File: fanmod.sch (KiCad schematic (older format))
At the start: 6 parts, among them J1 FAN_IN, J2 FAN_OUT, J4 COMM

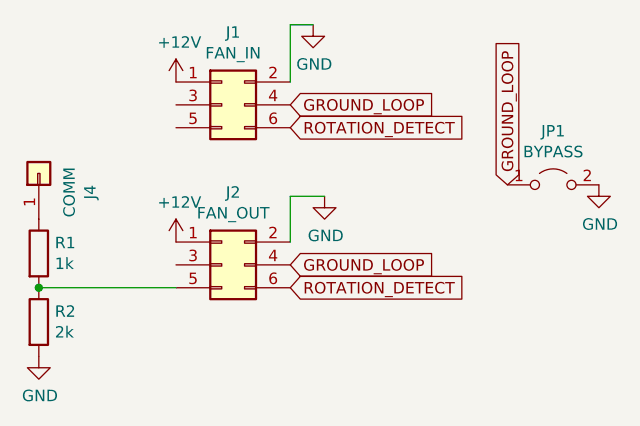
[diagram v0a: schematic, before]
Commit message: board v2.0
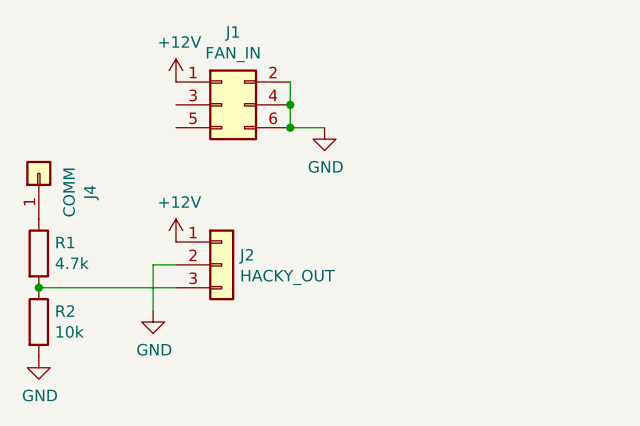
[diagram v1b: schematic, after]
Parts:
- removed J2: FAN_OUT, Connector_PinHeader_2.00mm:PinHeader_2x03_P2.00mm_Vertical_SMD, symbol Connector_Generic:Conn_02x03_Odd_Even
- removed JP1: BYPASS, Jumper:SolderJumper-2_P1.3mm_Open_RoundedPad1.0x1.5mm, symbol Jumper:Jumper_2_Open
- added J2: HACKY_OUT, Connector_PinHeader_2.00mm:PinHeader_1x03_P2.00mm_Vertical, symbol Connector_Generic:Conn_01x03
- J1: footprint Connector_PinSocket_2.00mm:PinSocket_2x03_P2.00mm_Vertical_SMD -> Connector_PinSocket_2.00mm:PinSocket_2x03_P2.00mm_Vertical
- R1: value 1k -> 4.7k
- R2: value 2k -> 10k
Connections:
- net GROUND_LOOP is gone; now on net GND: J1.4 (Pin_4)
- net ROTATION_DETECT is gone; now on net GND: J1.6 (Pin_6)
- net +12V: now also J2.1 (Pin_1)
- net GND: now also J2.2 (Pin_2)
- net at R1.2, R2.1: now also J2.3 (Pin_3)
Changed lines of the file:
@@
 $EndDescr
-$Comp
-L Connector_Generic:Conn_02x03_Odd_Even J2
-U 1 1 5E9E1E9C
-P 5350 3000
-F 0 "J2" H 5400 3317 50  0000 C CNN
-F 1 "FAN_OUT" H 5400 3226 50  0000 C CNN
-F 2 "Connector_PinHeader_2.00mm:PinHeader_2x03_P2.00mm_Vertical_SMD" H 5350 3000 50  0001 C CNN
-F 3 "~" H 5350 3000 50  0001 C CNN
-	1    5350 3000
-	1    0    0    -1
-$EndComp
-Wire Wire Line
-	5650 2700 5800 2700
-Wire Wire Line
-	5650 2900 5650 2700
-$Comp
-L power:GND #PWR0106
-U 1 1 5E9D0844
-P 5800 2700
-F 0 "#PWR0106" H 5800 2450 50  0001 C CNN
-F 1 "GND" H 5805 2527 50  0000 C CNN
-F 2 "" H 5800 2700 50  0001 C CNN
-F 3 "" H 5800 2700 50  0001 C CNN
-	1    5800 2700
-	1    0    0    -1
-$EndComp
 $Comp
 L power:+12V #PWR0105
@@
 	1    0    0    -1
 $EndComp
-Text GLabel 5650 3100 2    50   Input ~ 0
-ROTATION_DETECT
-Text GLabel 5650 2300 2    50   Input ~ 0
-GROUND_LOOP
-Text GLabel 5650 2400 2    50   Input ~ 0
-ROTATION_DETECT
-Wire Wire Line
-	5650 1950 5650 2200
 $Comp
 L Connector_Generic:Conn_02x03_Odd_Even J1
@@
 F 0 "J1" H 5400 2617 50  0000 C CNN
 F 1 "FAN_IN" H 5400 2526 50  0000 C CNN
-F 2 "Connector_PinSocket_2.00mm:PinSocket_2x03_P2.00mm_Vertical_SMD" H 5350 2300 50  0001 C CNN
+F 2 "Connector_PinSocket_2.00mm:PinSocket_2x03_P2.00mm_Vertical" H 5350 2300 50  0001 C CNN
 F 3 "~" H 5350 2300 50  0001 C CNN
 	1    5350 2300
 	1    0    0    -1
 $EndComp
-Wire Wire Line
-	5650 1950 5750 1950
 $Comp
 L power:GND #PWR0104
 U 1 1 5E9CC741
-P 5750 1950
-F 0 "#PWR0104" H 5750 1700 50  0001 C CNN
-F 1 "GND" H 5755 1777 50  0000 C CNN
-F 2 "" H 5750 1950 50  0001 C CNN
-F 3 "" H 5750 1950 50  0001 C CNN
-	1    5750 1950
+P 5800 2400
+F 0 "#PWR0104" H 5800 2150 50  0001 C CNN
+F 1 "GND" H 5805 2227 50  0000 C CNN
+F 2 "" H 5800 2400 50  0001 C CNN
+F 3 "" H 5800 2400 50  0001 C CNN
+	1    5800 2400
 	1    0    0    -1
 $EndComp
@@
 	0    -1   -1   0
 $EndComp
-Text GLabel 5650 3000 2    50   Input ~ 0
-GROUND_LOOP
-$Comp
-L Jumper:Jumper_2_Open JP1
-U 1 1 5EA1EF21
-P 6800 2650
-F 0 "JP1" H 6800 2885 50  0000 C CNN
-F 1 "BYPASS" H 6800 2794 50  0000 C CNN
-F 2 "Jumper:SolderJumper-2_P1.3mm_Open_RoundedPad1.0x1.5mm" H 6800 2650 50  0001 C CNN
-F 3 "~" H 6800 2650 50  0001 C CNN
-	1    6800 2650
-	1    0    0    -1
-$EndComp
-$Comp
-L power:GND #PWR0101
-U 1 1 5EA1F32A
-P 7000 2650
-F 0 "#PWR0101" H 7000 2400 50  0001 C CNN
-F 1 "GND" H 7005 2477 50  0000 C CNN
-F 2 "" H 7000 2650 50  0001 C CNN
-F 3 "" H 7000 2650 50  0001 C CNN
-	1    7000 2650
-	1    0    0    -1
-$EndComp
-Text GLabel 6600 2650 1    50   Input ~ 0
-GROUND_LOOP
 $Comp
 L Device:R R1
@@
 P 4550 2950
 F 0 "R1" H 4620 2996 50  0000 L CNN
-F 1 "1k" H 4620 2905 50  0000 L CNN
+F 1 "4.7k" H 4620 2905 50  0000 L CNN
 F 2 "Resistor_SMD:R_0603_1608Metric_Pad1.05x0.95mm_HandSolder" V 4480 2950 50  0001 C CNN
 F 3 "~" H 4550 2950 50  0001 C CNN
@@
 P 4550 3250
 F 0 "R2" H 4620 3296 50  0000 L CNN
-F 1 "2k" H 4620 3205 50  0000 L CNN
+F 1 "10k" H 4620 3205 50  0000 L CNN
 F 2 "Resistor_SMD:R_0603_1608Metric_Pad1.05x0.95mm_HandSolder" V 4480 3250 50  0001 C CNN
 F 3 "~" H 4550 3250 50  0001 C CNN
@@
 	5150 3100 4550 3100
 Connection ~ 4550 3100
+Wire Wire Line
+	5650 2400 5650 2300
+Connection ~ 5650 2400
+Wire Wire Line
+	5650 2200 5650 2300
+Connection ~ 5650 2300
+Wire Wire Line
+	5800 2400 5650 2400
+$Comp
+L Connector_Generic:Conn_01x03 J2
+U 1 1 5EE49454
+P 5350 3000
+F 0 "J2" H 5430 3042 50  0000 L CNN
+F 1 "HACKY_OUT" H 5430 2951 50  0000 L CNN
+F 2 "Connector_PinHeader_2.00mm:PinHeader_1x03_P2.00mm_Vertical" H 5350 3000 50  0001 C CNN
+F 3 "~" H 5350 3000 50  0001 C CNN
+	1    5350 3000
+	1    0    0    -1
+$EndComp
+$Comp
+L power:GND #PWR0106
+U 1 1 5EE4996A
+P 5050 3200
+F 0 "#PWR0106" H 5050 2950 50  0001 C CNN
+F 1 "GND" H 5055 3027 50  0000 C CNN
+F 2 "" H 5050 3200 50  0001 C CNN
+F 3 "" H 5050 3200 50  0001 C CNN
+	1    5050 3200
+	1    0    0    -1
+$EndComp
+Wire Wire Line
+	5150 3000 5050 3000
+Wire Wire Line
+	5050 3000 5050 3200
 $EndSCHEMATC
